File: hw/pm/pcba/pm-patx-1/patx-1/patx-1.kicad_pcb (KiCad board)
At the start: 2 copper layers, 70 x 90 mm, 18 parts, among them J1 ATX-24, J10 Conn_01x08, J11 Conn_02x08_Top_Bottom, J12 Conn_02x08_Top_Bottom, J13 Conn_02x08_Top_Bottom, J14 Conn_02x08_Top_Bottom, J15 Conn_02x08_Top_Bottom, J2 Conn_01x02, J3 Conn_01x02, J4 Conn_01x02, J5 Conn_01x02, J6 USB_A, J7 USB_A, J8 USB_A, J9 USB_A, SW1 SW_SPDT

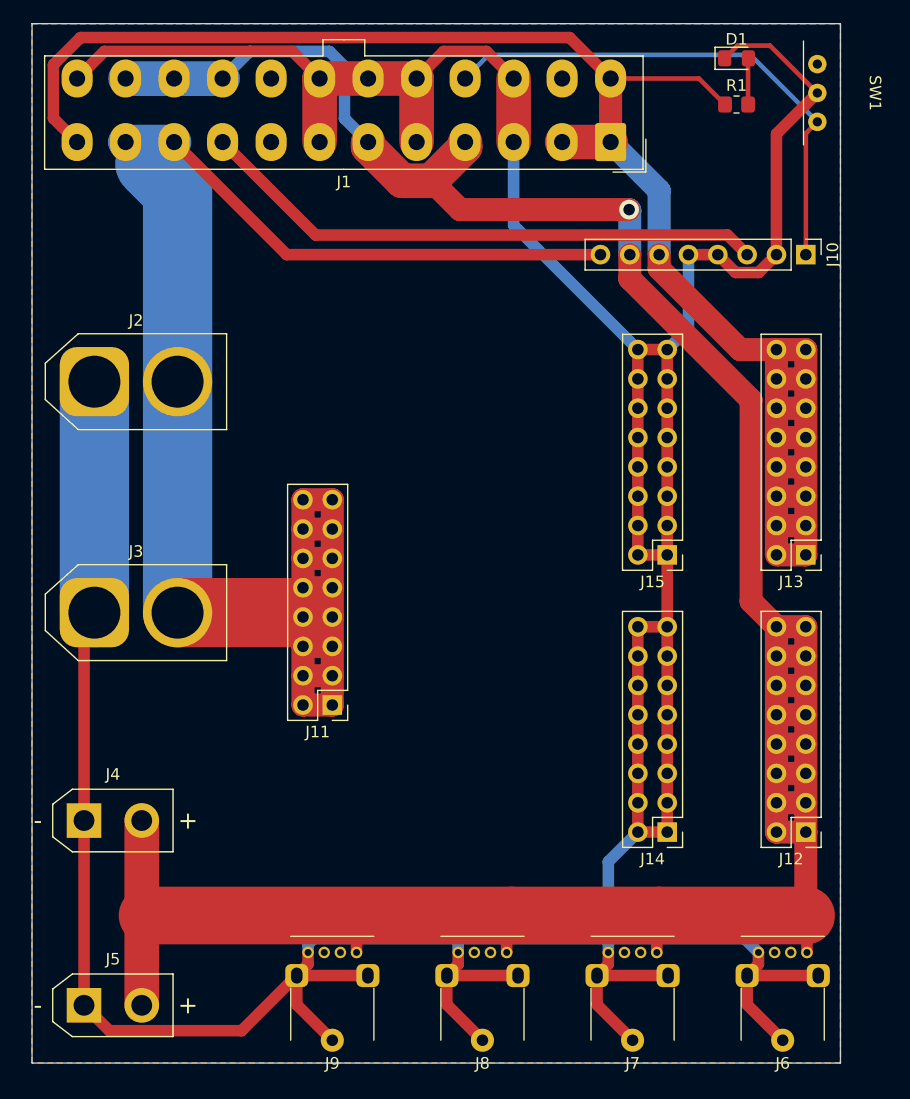
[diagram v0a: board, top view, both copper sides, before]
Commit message: 添加(pm/pcba): pm-patx-1
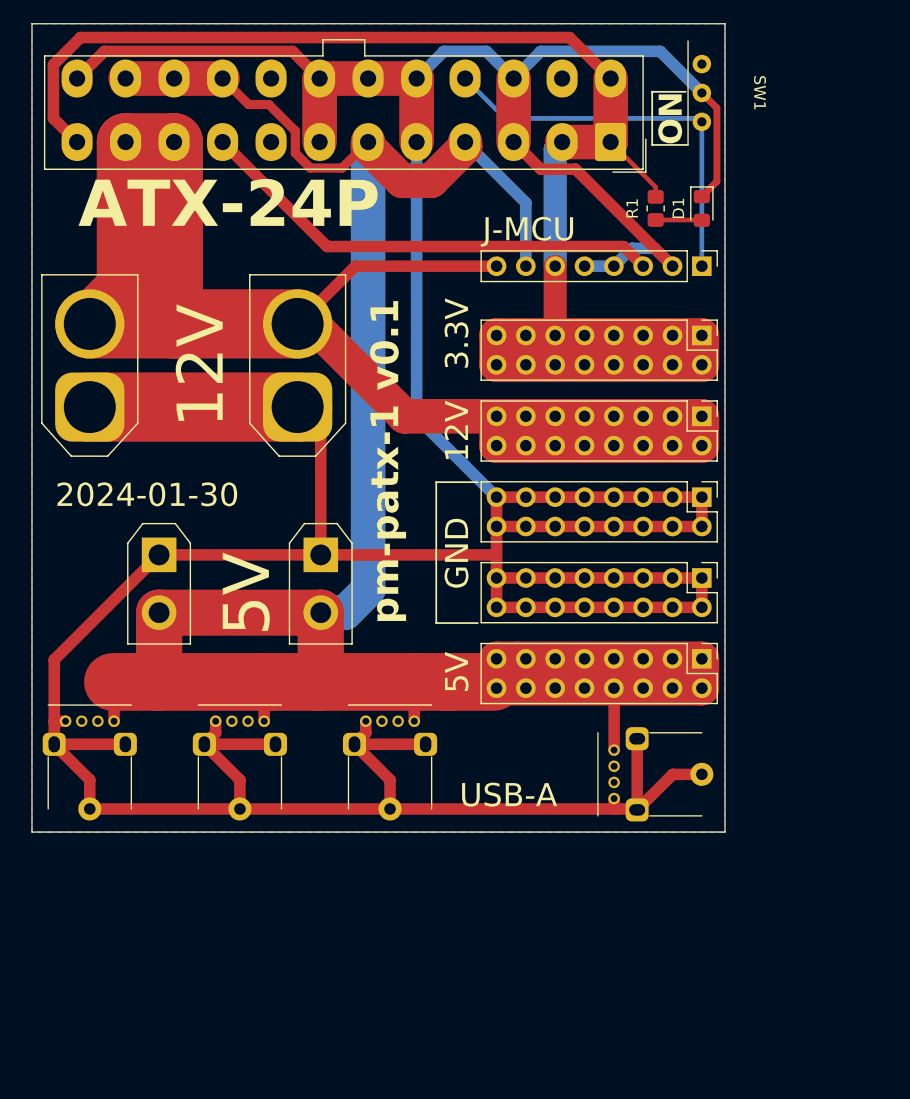
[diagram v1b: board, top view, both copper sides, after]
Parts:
- moved J5 44.1 mm to (64.0, 85.0), turned to -90 degrees
- moved J11 40.6 mm to (97.0, 73.0), turned to -90 degrees
- moved J6 39.5 mm to (70.0, 107.0)
- moved J7 39.5 mm to (57.0, 107.0)
- moved J8 39.5 mm to (44.0, 107.0)
- moved J9 39.4 mm to (97.0, 104.0), turned to 90 degrees
- moved J14 29.2 mm to (97.0, 80.0), turned to -90 degrees
- moved J3 25.0 mm to (62.0, 72.2), turned to 90 degrees
- moved J4 23.9 mm to (50.0, 85.0), turned to -90 degrees
- moved J13 21.0 mm to (97.0, 66.0), turned to -90 degrees
- moved J12 17.5 mm to (97.0, 94.0), turned to -90 degrees
- moved D1 13.3 mm to (97.0, 55.0), turned to -90 degrees
- moved R1 11.4 mm to (93.0, 55.0), turned to -90 degrees
- moved SW1 10.0 mm to (97.0, 45.0)
- moved J10 9.06 mm to (97.0, 60.0)
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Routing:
- net +5V: track 248.7 -> 210.1 mm, vias 1 -> 0
- net +3.3V: track 160.3 -> 131.9 mm
- net +12V: track 161.4 -> 135.4 mm
- net GND: track 402.2 -> 420.8 mm
- net /PS_ON: track 45.7 -> 34.6 mm
- net /5VSB: track 49.5 -> 40.9 mm
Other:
- board size 70 x 90 mm -> 60 x 70 mm
- board text added: "+12V"
- board text added: "+5V"
- board text added: "12V"
- board text added: "2024-01-30"
- board text added: "3.3V"
- board text added: "5V"
- board text added: "ATX-24P"
- board text added: "GND"
- board text added: "J-MCU"
- board text added: "ON"
- board text added: "USB-A"
- board text added: "pm-patx-1 v0.1"
